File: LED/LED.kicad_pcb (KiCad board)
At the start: 2 copper layers, 64.6 x 61.9 mm, 23 parts, among them J1 USB_C_Receptacle_USB2.0, J2 RJ45, SW1 SW_Push, U1 CH340C, U2 WeMos_D1_mini, U3 ESP32-WROOM-32D, U4 AMS1117-3.3

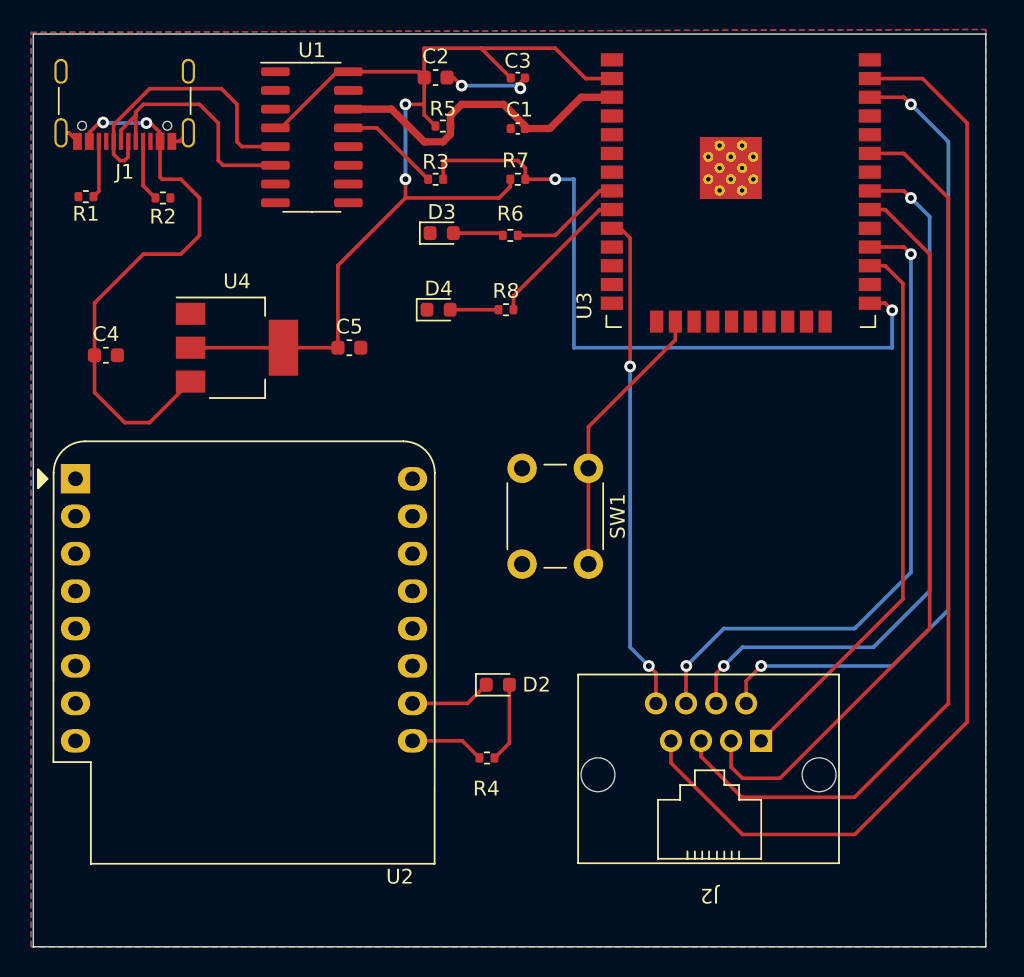
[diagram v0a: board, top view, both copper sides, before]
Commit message: Routing Done
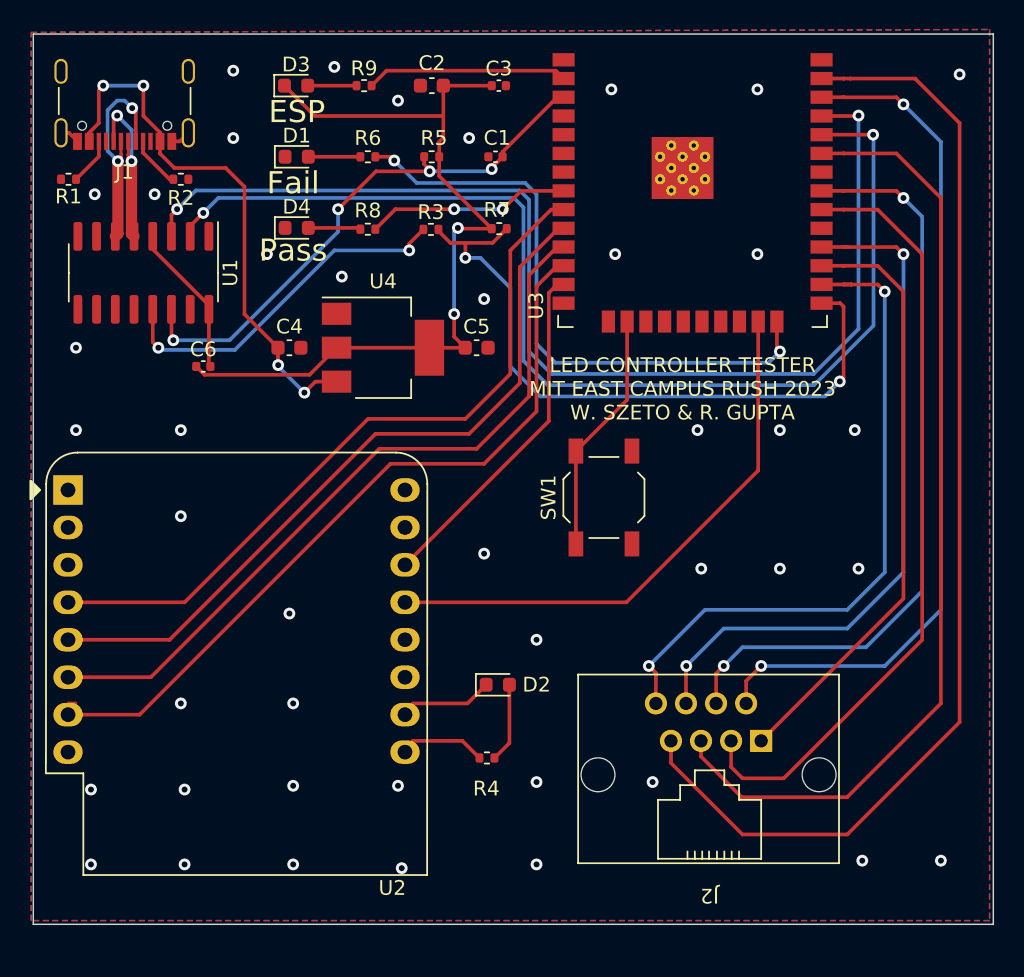
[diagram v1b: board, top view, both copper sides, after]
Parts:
- added C6: 100nF, Capacitor_SMD:C_0402_1005Metric, F.Cu at (81.5, 82.5)
- added D1: R_LED, LED_SMD:LED_0603_1608Metric, F.Cu at (87.9, 68.3)
- added R9: 1K, Resistor_SMD:R_0402_1005Metric, F.Cu at (92.4, 63.5)
- D3: value R_LED -> LED
- SW1: footprint Button_Switch_THT:SW_PUSH_6mm -> Button_Switch_SMD:SW_SPST_TL3342
- moved U1 14.7 mm to (77.5, 76.2), turned to -90 degrees
- moved D3 14.1 mm to (87.8, 63.5)
- moved C4 12.5 mm to (87.4, 81.3)
- moved D4 11.1 mm to (87.9, 73.2)
- moved R6 11.0 mm to (92.7, 68.3)
- moved R8 10.8 mm to (92.7, 73.2)
- moved U4 9.91 mm to (93.7, 81.3)
- moved C5 8.64 mm to (100.1, 81.3)
- moved R7 3.58 mm to (101.6, 73.2)
- moved R3 3.42 mm to (97.0, 73.3)
- moved U3 3.27 mm to (114.7, 70.0)
- moved C1 2.44 mm to (101.4, 68.3)
- moved SW1 2.24 mm to (108.7, 91.4), turned to 90 degrees
- moved R5 2.22 mm to (97.0, 68.3), turned to 180 degrees
- moved R2 1.76 mm to (80.0, 69.8)
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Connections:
- D3 pad 1: GND -> +3.3V
- R6 pad 1: Net-(R6-Pad1) -> Net-(U3-Pad24)
- R6 pad 2: Net-(D3-Pad2) -> Net-(D1-Pad2)
- R8 pad 1: Net-(R8-Pad1) -> Net-(U3-Pad8)
- U1 pad 16: +3.3V -> Net-(U1-Pad16)
- U1 pad 4: +3.3V -> Net-(U1-Pad16)
- U3 pad 10: /PIN8_GOOD -> /B_SIG
- U3 pad 11: unconnected-(U3-Pad11) -> /R_SIG
- U3 pad 12: unconnected-(U3-Pad12) -> /G_SIG
- U3 pad 13: unconnected-(U3-Pad13) -> /ARGB2
- U3 pad 2: +3.3V -> Net-(U3-Pad2)
- U3 pad 23: unconnected-(U3-Pad23) -> /ARGB1
- U3 pad 24: unconnected-(U3-Pad24) -> Net-(U3-Pad24)
- U3 pad 26: unconnected-(U3-Pad26) -> /PIN8_GOOD
- U3 pad 34: unconnected-(U3-Pad34) -> /TXD
- U3 pad 35: unconnected-(U3-Pad35) -> /RXD
- U3 pad 8: Net-(R6-Pad1) -> Net-(U3-Pad8)
- U3 pad 9: Net-(R8-Pad1) -> /W_SIG
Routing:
- net /RXD: track 0.00 -> 78.2 mm, vias 0 -> 2
- net /TXD: track 0.00 -> 77.3 mm, vias 0 -> 2
- net /G_SIG: track 0.00 -> 51.7 mm
- net /R_SIG: track 0.00 -> 50.5 mm
- net /B_SIG: track 0.00 -> 50.4 mm
- net /W_SIG: track 0.00 -> 49.6 mm
- net Net-(U3-Pad24): track 0.00 -> 41.6 mm, vias 0 -> 2
- net /ARGB1: track 0.00 -> 37.8 mm
- net /ARGB2: track 0.00 -> 23.7 mm
- net Net-(R3-Pad1): track 6.85 -> 24.5 mm, vias 0 -> 2
- net /RST: track 22.3 -> 37.9 mm, vias 0 -> 4
- net +3.3V: track 71.5 -> 56.3 mm
- net Net-(U3-Pad8): track 0.00 -> 13.8 mm, vias 0 -> 2
- net Net-(U3-Pad2): track 0.00 -> 13.7 mm
- net /PIN8_GOOD: track 33.8 -> 45.4 mm
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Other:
- board size 64.6 x 61.9 mm -> 65.1 x 60.4 mm
- board text added: "ESP"
- board text added: "LED CONTROLLER TESTER MIT EAST CAMPUS RUSH 2023 W. SZETO & R. GUPTA"
